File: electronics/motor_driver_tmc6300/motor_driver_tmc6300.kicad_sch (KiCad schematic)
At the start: 56 parts, among them IC1 TMC6300, U1 U, U2 U, U3 U, U4 U

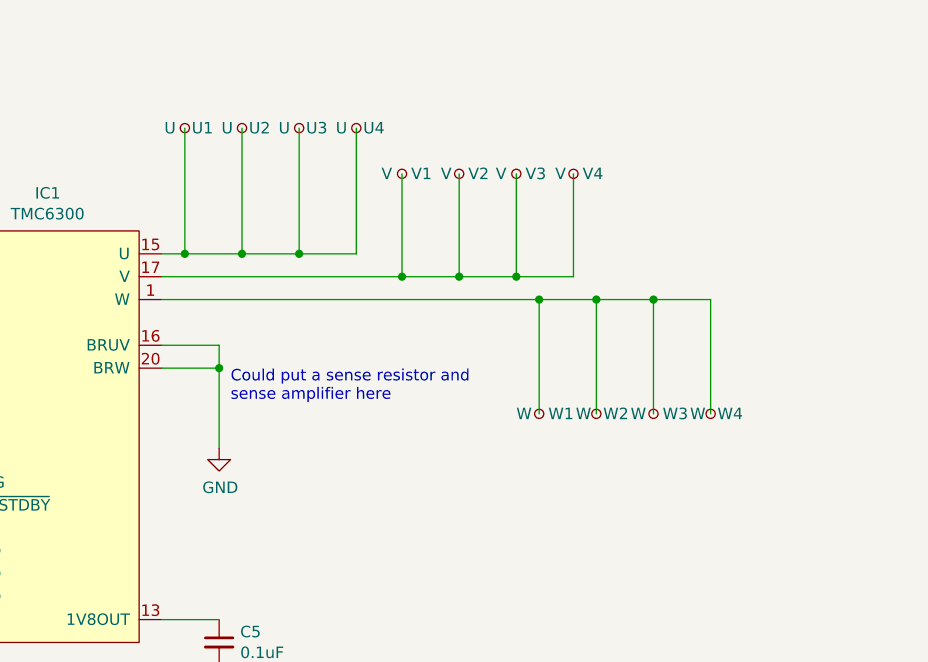
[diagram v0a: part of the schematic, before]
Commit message: update
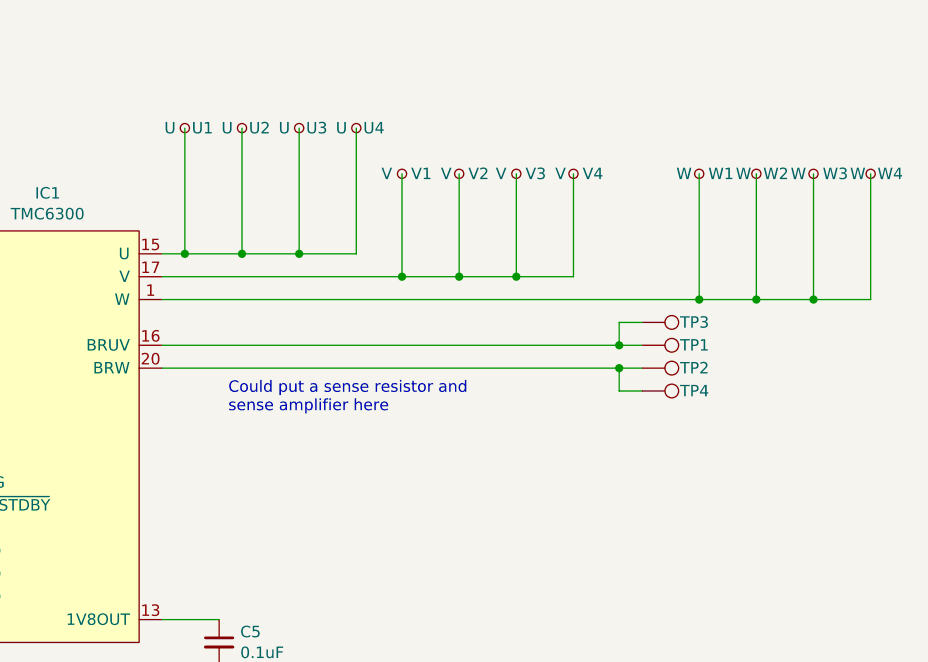
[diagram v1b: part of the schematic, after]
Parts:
- added TP1, TP2, TP3, TP4: TestPoint, Library:kawashima_TestPoint_THTPad_D1.5mm_Drill0.7mm, symbol Connector:TestPoint
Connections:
- net GND: no longer IC1.16 (BRUV), IC1.20 (BRW)
- new net: IC1.16 (BRUV), TP1.1, TP3.1
- new net: IC1.20 (BRW), TP2.1, TP4.1
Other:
- moved on the sheet: W1, W2, W3, W4
